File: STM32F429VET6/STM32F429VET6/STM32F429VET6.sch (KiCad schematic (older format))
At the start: 28 parts

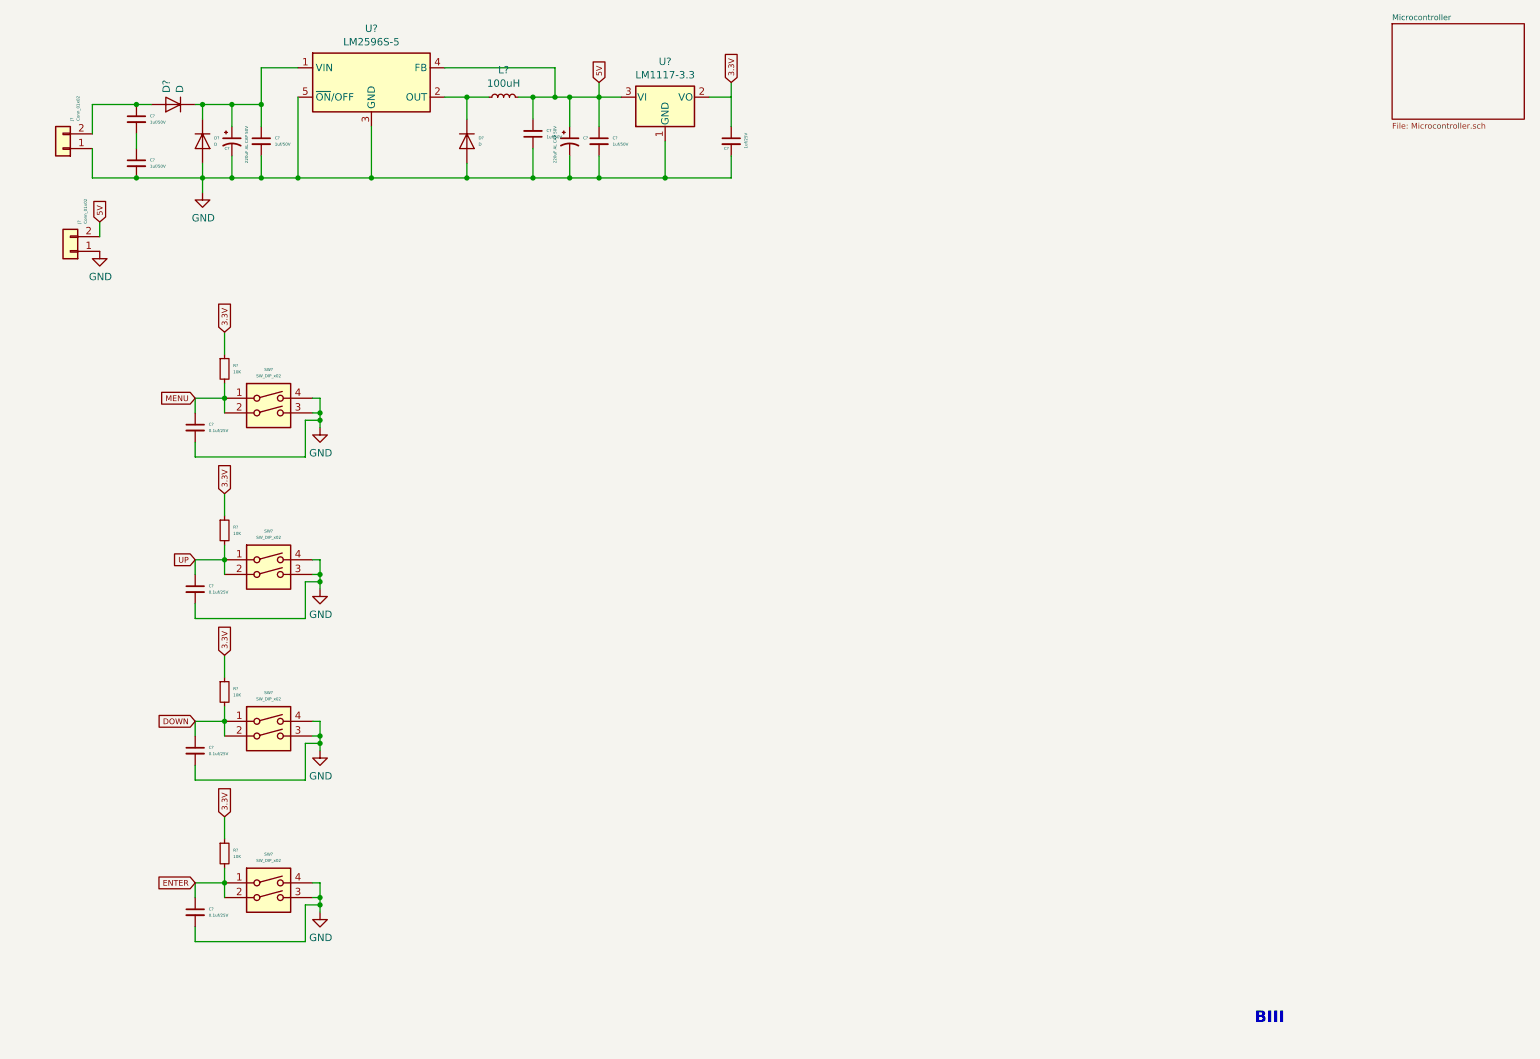
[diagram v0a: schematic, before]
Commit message: Completed 2 sections
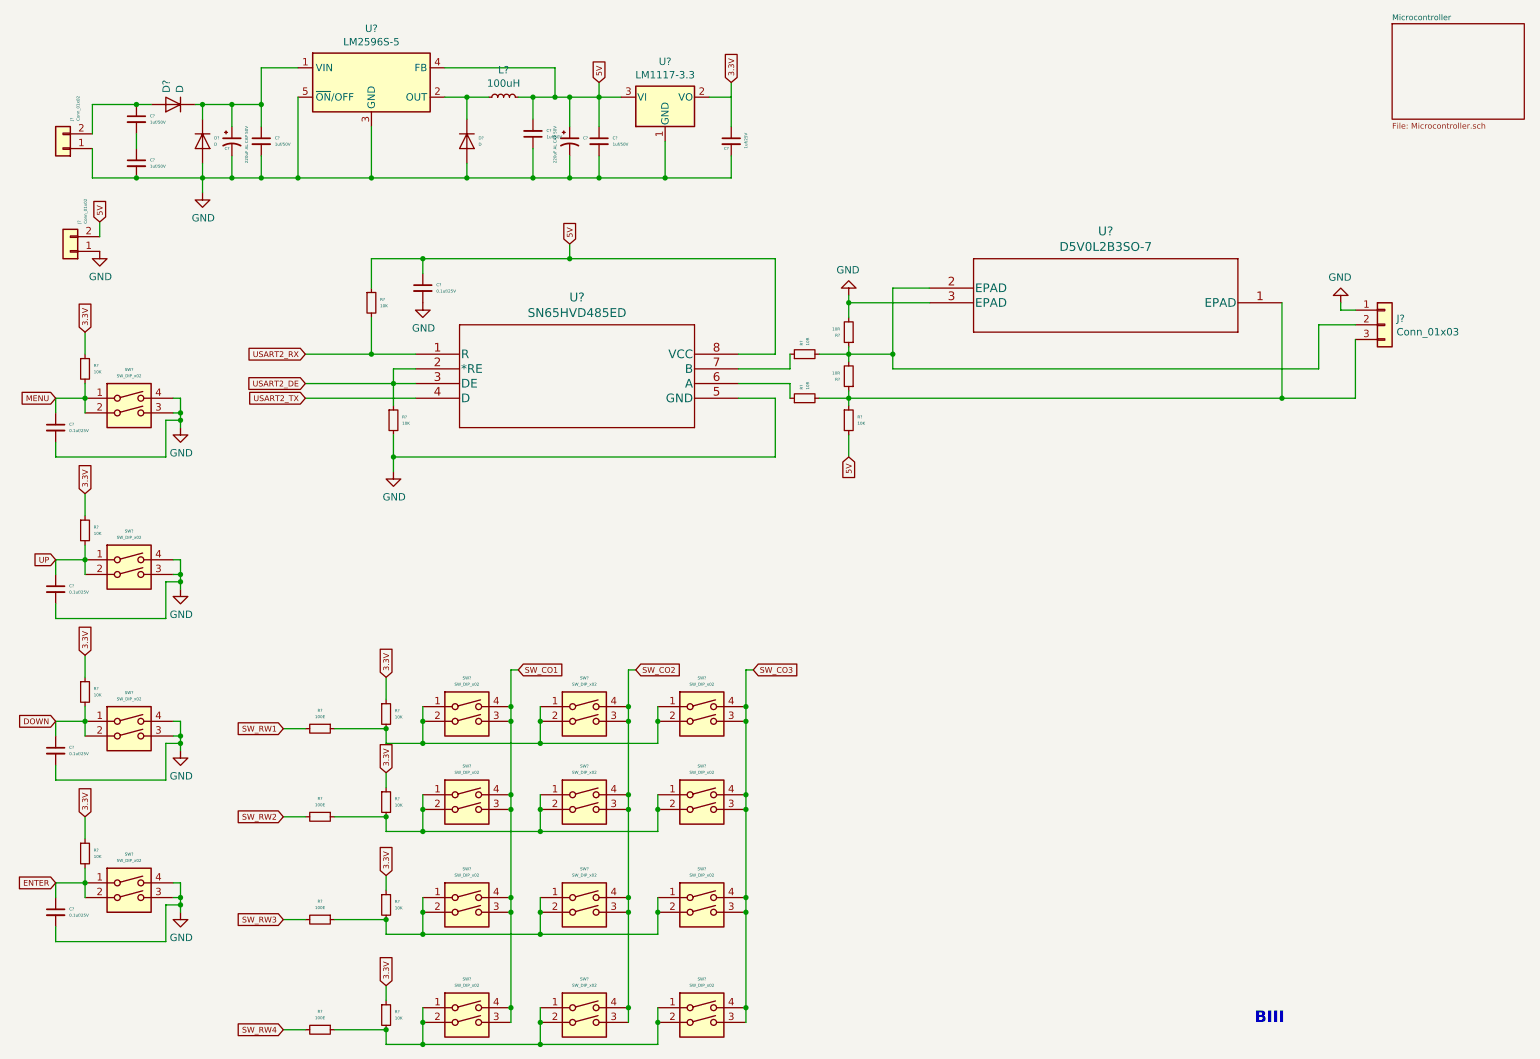
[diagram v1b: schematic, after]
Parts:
- added C?: 0.1uf/25V, Capacitor_SMD:C_0805_2012Metric_Pad1.15x1.40mm_HandSolder, symbol Device:C_Small
- added J?: Conn_01x03, symbol Connector_Generic:Conn_01x03
- added R? (x7): 10K, Resistor_SMD:R_0805_2012Metric_Pad1.15x1.40mm_HandSolder, symbol Device:R_Small
- added R? (x4): 100E, Resistor_SMD:R_0805_2012Metric_Pad1.15x1.40mm_HandSolder, symbol Device:R_Small
- added R? (x4): 10R, Resistor_SMD:R_0805_2012Metric_Pad1.15x1.40mm_HandSolder, symbol Device:R_Small
- added SW? (x12): SW_DIP_x02, Button_Switch_SMD:SW_SPST_B3S-1000, symbol Switch:SW_DIP_x02
- added U?: SN65HVD485ED, SN65HVD485ED:SN65HVD485ED, symbol SN65HVD485ED:SN65HVD485ED
- added U?: D5V0L2B3SO-7, D5V0L2B3SO7:D5V0L2B3SO-7, symbol D5V0L2B3SO7:D5V0L2B3SO-7
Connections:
- net 3.3V: now also R?.1, R?.1, R?.1, R?.1
- net 5V: now also C?.1, R?.1, R?.2, U?.8 (VCC)
- net GND: now also C?.2, J?.1 (Pin_1), R?.2, R?.2, U?.3 (EPAD), U?.5 (GND)
- new net: R?.1, R?.2, SW?.1, SW?.1, SW?.1, SW?.2, SW?.2, SW?.2 (x4)
- new net: R?.1, U?.6 (A)
- new net: R?.1, U?.7 (B)
- new net: J?.3 (Pin_3), R?.1, R?.1, R?.2, U?.1 (EPAD)
- new net: J?.2 (Pin_2), R?.1, R?.2, R?.2, U?.2 (EPAD)
- new net SW_CO1: SW?.3, SW?.3, SW?.3, SW?.3, SW?.4, SW?.4, SW?.4, SW?.4
- new net SW_CO2: SW?.3, SW?.3, SW?.3, SW?.3, SW?.4, SW?.4, SW?.4, SW?.4
- new net SW_CO3: SW?.3, SW?.3, SW?.3, SW?.3, SW?.4, SW?.4, SW?.4, SW?.4
- new net SW_RW1: R?.2
- new net SW_RW2: R?.2
- new net SW_RW3: R?.2
- new net SW_RW4: R?.2
- new net USART2_DE: R?.1, U?.2 (*RE), U?.3 (DE)
- new net USART2_RX: R?.2, U?.1 (R)
- new net USART2_TX: U?.4 (D)
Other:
- moved on the sheet: C?, R?, SW?
